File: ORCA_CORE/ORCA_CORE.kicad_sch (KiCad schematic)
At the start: 6 parts, among them J17 Vin_motor, J18 data_line_power, J19 +5Vin_cpu, J23 motor_fork, J24 motor_arm, J25 servo_arm

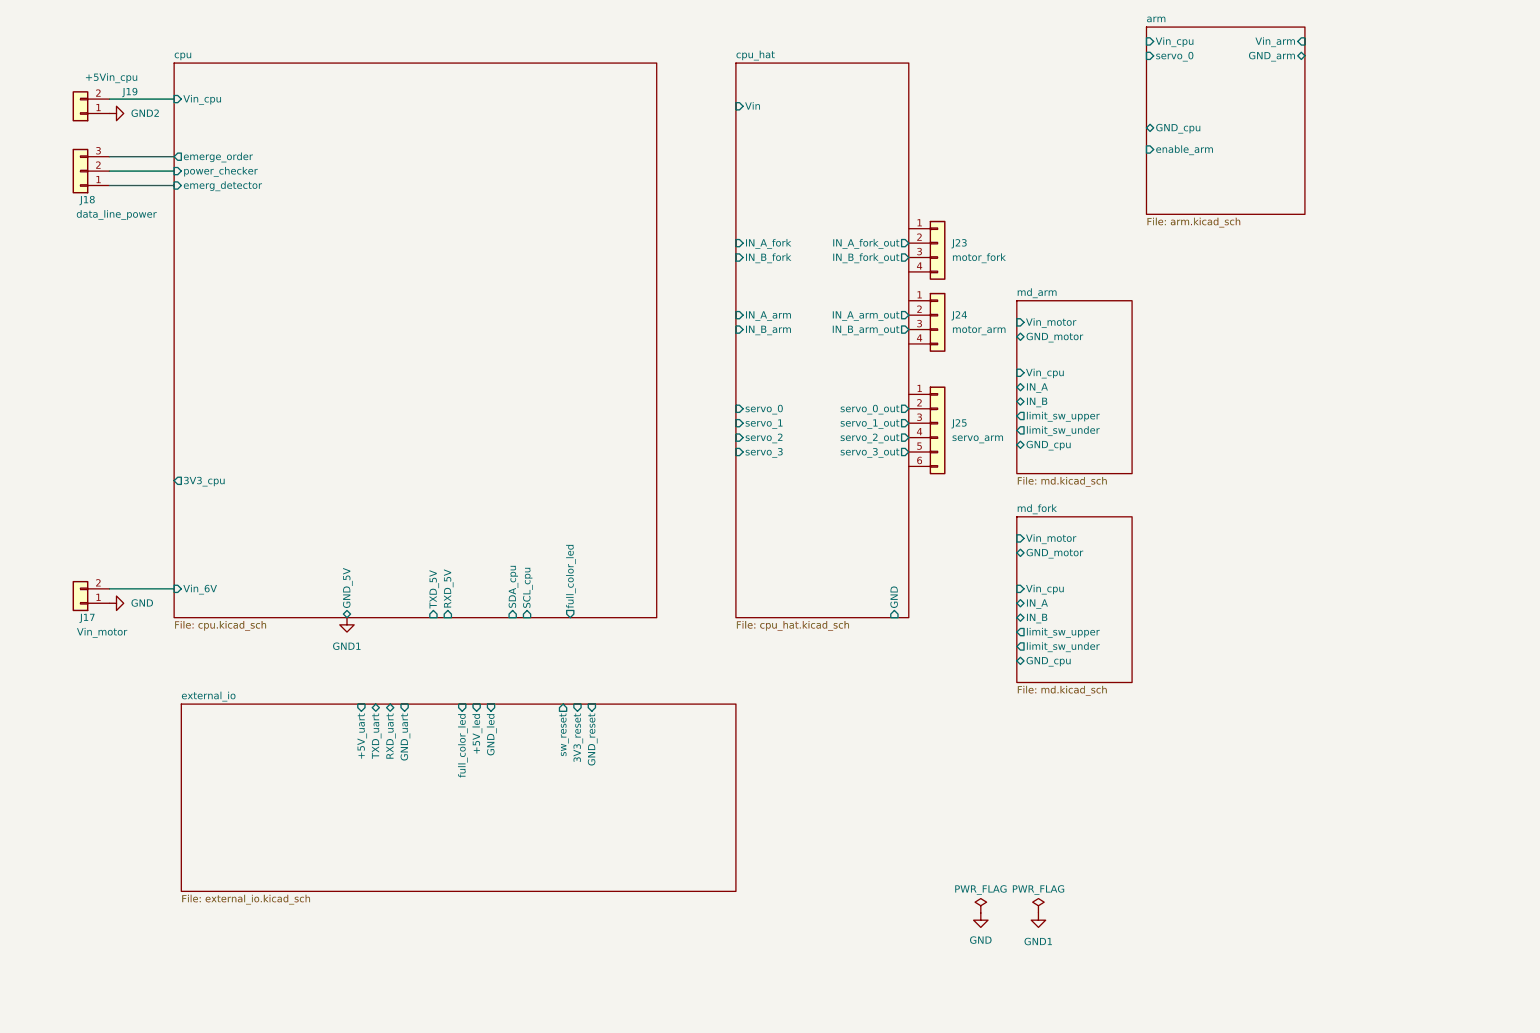
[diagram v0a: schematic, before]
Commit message: almost completed CORE
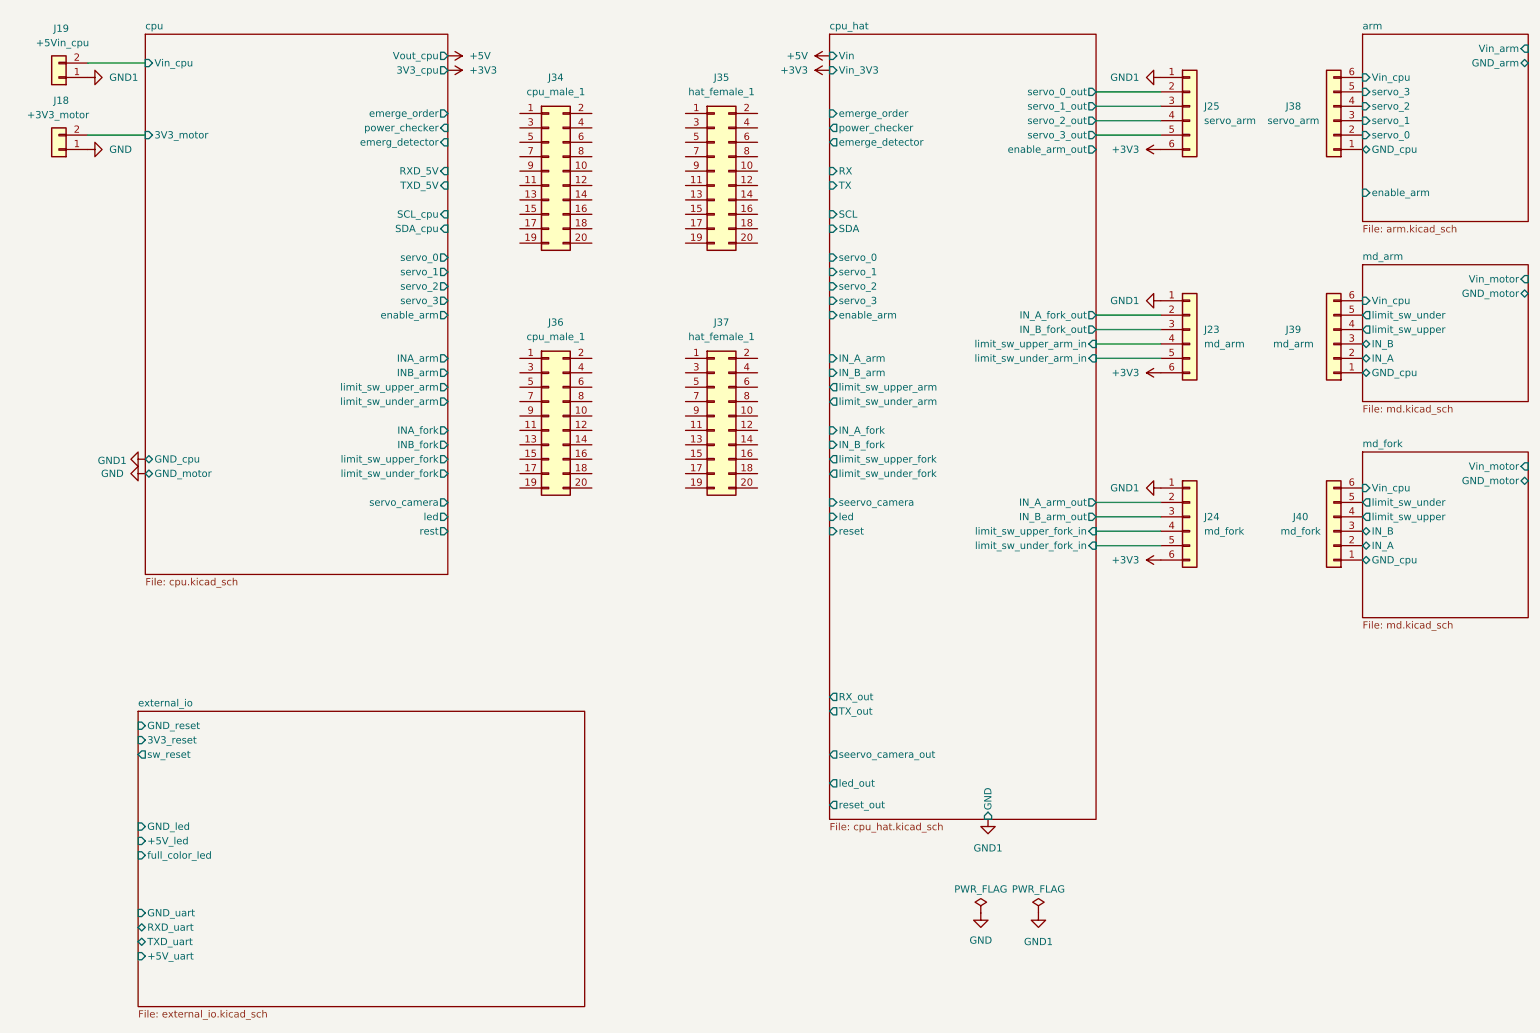
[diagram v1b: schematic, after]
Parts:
- removed J17: Vin_motor, Conn:power_pad, symbol Connector_Generic:Conn_01x02
- removed J18: data_line_power, Connector_JST:JST_XH_B3B-XH-A_1x03_P2.50mm_Vertical, symbol Connector_Generic:Conn_01x03
- removed J23: motor_fork, symbol Connector_Generic:Conn_01x04
- removed J24: motor_arm, symbol Connector_Generic:Conn_01x04
- added J18: +3V3_motor, Conn:power_pad, symbol Connector_Generic:Conn_01x02
- added J23, J39: md_arm, symbol Connector_Generic:Conn_01x06
- added J24, J40: md_fork, symbol Connector_Generic:Conn_01x06
- added J34, J36: cpu_male_1, Connector_PinHeader_2.54mm:PinHeader_2x10_P2.54mm_Vertical, symbol Connector_Generic:Conn_02x10_Odd_Even
- added J35, J37: hat_female_1, Connector_PinHeader_2.54mm:PinHeader_2x10_P2.54mm_Vertical, symbol Connector_Generic:Conn_02x10_Odd_Even
- added J38: servo_arm, symbol Connector_Generic:Conn_01x06
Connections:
- net GND2 is gone; now on net GND1: J19.1 (Pin_1)
- net GND: now also J18.1 (Pin_1)
- net GND1: now also J25.1 (Pin_1), J23.1 (Pin_1), J24.1 (Pin_1)
- net arm/GND_cpu: now also J38.1 (Pin_1)
- net arm/Vin_cpu: now also J38.6 (Pin_6)
- net arm/servo_0: now also J38.2 (Pin_2)
- net cpu_hat/IN_A_arm_out: now also J24.2 (Pin_2)
- net cpu_hat/IN_A_fork_out: now also J23.2 (Pin_2)
- net cpu_hat/IN_B_arm_out: now also J24.3 (Pin_3)
- net cpu_hat/IN_B_fork_out: now also J23.3 (Pin_3)
- net md_arm/GND_cpu: now also J39.1 (Pin_1)
- net md_arm/IN_A: now also J39.2 (Pin_2)
- net md_arm/IN_B: now also J39.3 (Pin_3)
- net md_arm/Vin_cpu: now also J39.6 (Pin_6)
- net md_arm/limit_sw_under: now also J39.5 (Pin_5)
- net md_arm/limit_sw_upper: now also J39.4 (Pin_4)
- net md_fork/GND_cpu: now also J40.1 (Pin_1)
- net md_fork/IN_A: now also J40.2 (Pin_2)
- net md_fork/IN_B: now also J40.3 (Pin_3)
- net md_fork/Vin_cpu: now also J40.6 (Pin_6)
- net md_fork/limit_sw_under: now also J40.5 (Pin_5)
- net md_fork/limit_sw_upper: now also J40.4 (Pin_4)
- net +3V3: now reaches J25.6 (Pin_6)
- net +3V3: now also J23.6 (Pin_6), J24.6 (Pin_6)
- new net arm/servo_1: J38.3 (Pin_3)
- new net arm/servo_2: J38.4 (Pin_4)
- new net arm/servo_3: J38.5 (Pin_5)
- new net cpu/3V3_motor: J18.2 (Pin_2)
- new net cpu_hat/limit_sw_under_arm_in: J23.5 (Pin_5)
- new net cpu_hat/limit_sw_under_fork_in: J24.5 (Pin_5)
- new net cpu_hat/limit_sw_upper_arm_in: J23.4 (Pin_4)
- new net cpu_hat/limit_sw_upper_fork_in: J24.4 (Pin_4)
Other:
- sheet arm ports: added servo_1, servo_2, servo_3; removed none
- sheet cpu ports: added 3V3_motor, GND_cpu, GND_motor, INA_arm, INA_fork, INB_arm, INB_fork, Vout_cpu, enable_arm, led, limit_sw_under_arm, limit_sw_under_fork, limit_sw_upper_arm, limit_sw_upper_fork, rest, servo_0, servo_1, servo_2, servo_3, servo_camera; removed GND_5V, Vin_6V, full_color_led
- sheet cpu_hat ports: added RX, RX_out, SCL, SDA, TX, TX_out, Vin_3V3, emerge_detector, emerge_order, enable_arm, enable_arm_out, led, led_out, limit_sw_under_arm, limit_sw_under_arm_in, limit_sw_under_fork, limit_sw_under_fork_in, limit_sw_upper_arm, limit_sw_upper_arm_in, limit_sw_upper_fork, limit_sw_upper_fork_in, power_checker, reset, reset_out, seervo_camera, seervo_camera_out; removed none
- moved on the sheet: J19, J25
